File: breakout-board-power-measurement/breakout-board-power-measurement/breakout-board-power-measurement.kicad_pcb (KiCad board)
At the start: 2 copper layers, 70.6 x 40.2 mm, 83 parts, among them J1 Screw_Terminal_01x04, J2 Conn_01x09, J3 Conn_01x07, J4 Conn_01x02, U1 MCP3911A0-E-SS, U2 Si8641BA-B-IU, U3 LM317_TO-252, Y1 10M

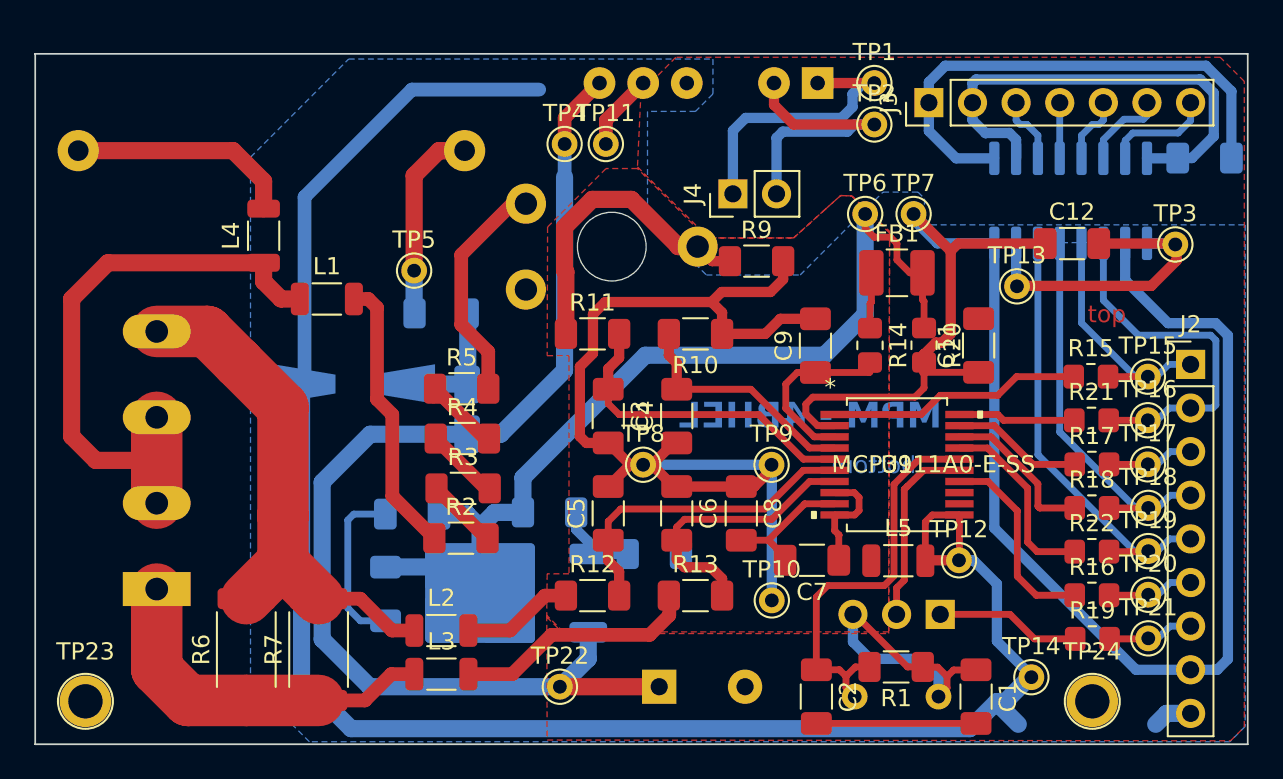
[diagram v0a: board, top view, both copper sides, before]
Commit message: Minor Fixes.
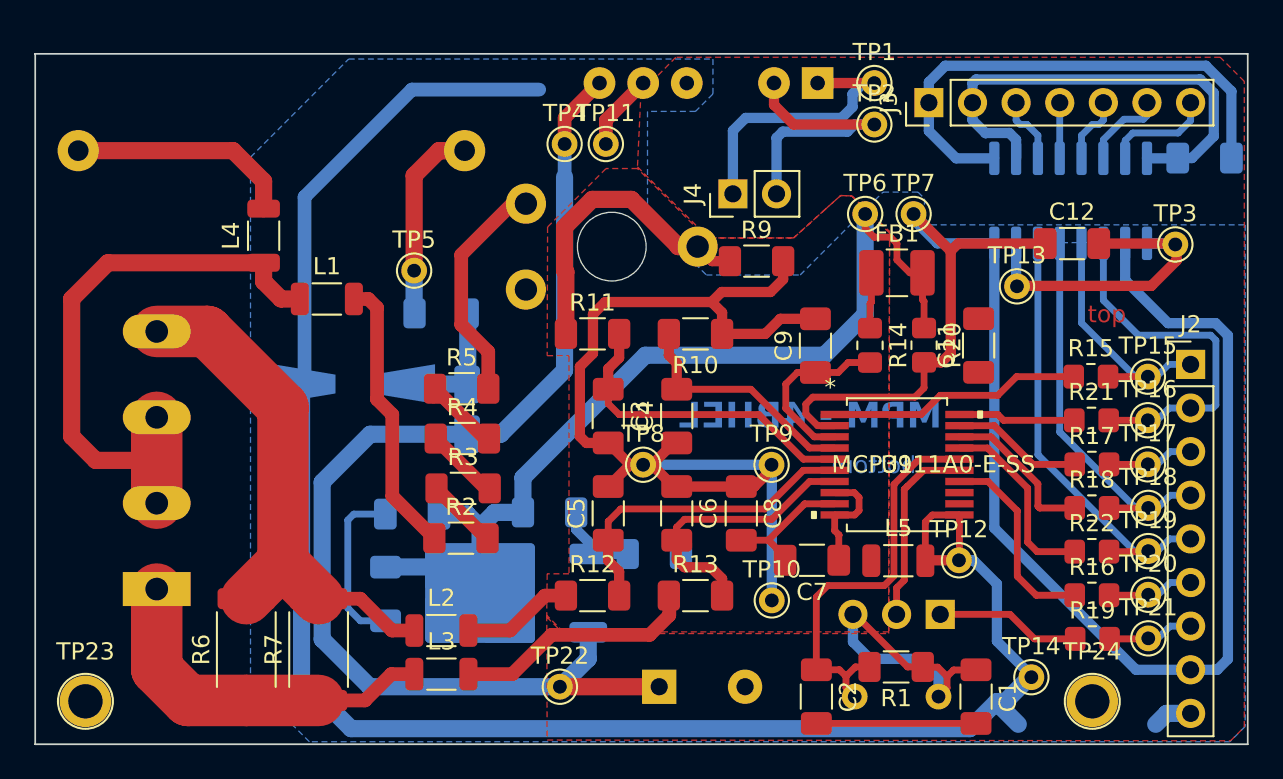
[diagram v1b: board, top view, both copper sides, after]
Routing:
- net /3V3D: track 98.8 -> 95.1 mm
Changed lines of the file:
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@@
   (segment (start 167.8432 143.5608) (end 168.402 143.002) (width 0.4) (layer "F.Cu") (net 9))
   (segment (start 162.1028 131.826) (end 162.7755 131.1533) (width 0.4) (layer "F.Cu") (net 10))
-  (segment (start 163.83 131.153298) (end 166.976701 131.153298) (width 0.4) (layer "F.Cu") (net 10))
+  (segment (start 165.736534 130.573466) (end 167.006533 130.573466) (width 0.4) (layer "F.Cu") (net 10))
+  (segment (start 165.156702 131.153298) (end 165.736534 130.573466) (width 0.4) (layer "F.Cu") (net 10))
+  (segment (start 163.83 131.153298) (end 165.156702 131.153298) (width 0.4) (layer "F.Cu") (net 10))
   (segment (start 164.9476 134.899999) (end 163.756198 134.899999) (width 0.4) (layer "F.Cu") (net 10))
   (segment (start 163.756198 134.899999) (end 162.1028 133.246601) (width 0.4) (layer "F.Cu") (net 10))
@@
   (segment (start 163.829998 131.1533) (end 163.83 131.153298) (width 0.4) (layer "F.Cu") (net 10))
   (segment (start 162.7755 131.1533) (end 163.829998 131.1533) (width 0.4) (layer "F.Cu") (net 10))
-  (segment (start 166.976701 131.153298) (end 167.006533 131.123466) (width 0.4) (layer "F.Cu") (net 10))
-  (segment (start 170.153066 130.074934) (end 170.178592 130.074934) (width 0.6) (layer "F.Cu") (net 11))
-  (segment (start 171.704 128.905) (end 171.704 124.084) (width 0.6) (layer "F.Cu") (net 11))
-  (segment (start 173.3296 131.144632) (end 170.182898 131.144632) (width 0.4) (layer "F.Cu") (net 11))
+  (segment (start 171.704 124.084) (end 171.704 130.016) (width 0.6) (layer "F.Cu") (net 11))
   (segment (start 169.6212 132.588) (end 170.153066 132.056134) (width 0.4) (layer "F.Cu") (net 11))
   (segment (start 164.9476 134.250001) (end 163.954728 134.250001) (width 0.4) (layer "F.Cu") (net 11))
+  (segment (start 170.153066 132.056134) (end 170.153066 130.5648) (width 0.4) (layer "F.Cu") (net 11))
+  (segment (start 171.704 130.016) (end 171.1552 130.5648) (width 0.6) (layer "F.Cu") (net 11))
   (segment (start 163.6776 132.588) (end 169.6212 132.588) (width 0.4) (layer "F.Cu") (net 11))
-  (segment (start 170.182898 131.144632) (end 170.153066 131.1148) (width 0.4) (layer "F.Cu") (net 11))
   (segment (start 172.1408 123.6472) (end 171.704 124.084) (width 0.6) (layer "F.Cu") (net 11))
-  (segment (start 170.840526 129.413) (end 171.196 129.413) (width 0.6) (layer "F.Cu") (net 11))
   (segment (start 163.2712 133.566473) (end 163.2712 132.9944) (width 0.4) (layer "F.Cu") (net 11))
   (segment (start 171.704 124.084) (end 169.545 121.925) (width 0.6) (layer "F.Cu") (net 11))
   (segment (start 163.954728 134.250001) (end 163.2712 133.566473) (width 0.4) (layer "F.Cu") (net 11))
   (segment (start 177.2027 123.6472) (end 172.1408 123.6472) (width 0.6) (layer "F.Cu") (net 11))
-  (segment (start 170.153066 131.1148) (end 170.153066 130.074934) (width 0.6) (layer "F.Cu") (net 11))
-  (segment (start 171.196 129.413) (end 171.704 128.905) (width 0.6) (layer "F.Cu") (net 11))
-  (segment (start 170.178592 130.074934) (end 170.840526 129.413) (width 0.6) (layer "F.Cu") (net 11))
   (segment (start 163.2712 132.9944) (end 163.6776 132.588) (width 0.4) (layer "F.Cu") (net 11))
-  (segment (start 170.153066 132.056134) (end 170.153066 131.1148) (width 0.4) (layer "F.Cu") (net 11))
+  (segment (start 171.1552 130.5648) (end 170.153066 130.5648) (width 0.6) (layer "F.Cu") (net 11))
   (segment (start 170.9278 123.633) (end 174.244 123.633) (width 0.6) (layer "B.Cu") (net 11))
   (segment (start 182.499 148.463) (end 174.244 140.208) (width 0.6) (layer "B.Cu") (net 11))
   (segment (start 187.8472 147.8392) (end 187.2234 148.463) (width 0.6) (layer "B.Cu") (net 11))
-  (segment (start 169.5704 121.4628) (end 169.5704 122.2756) (width 0.6) (layer "B.Cu") (net 11))
   (segment (start 181.864 125.7808) (end 184.3644 128.2812) (width 0.6) (layer "B.Cu") (net 11))
   (segment (start 169.5704 122.2756) (end 170.9278 123.633) (width 0.6) (layer "B.Cu") (net 11))
@@
   (segment (start 134.9 144.325) (end 137.325 144.325) (width 0.8) (layer "F.Cu") (net 36))
   (segment (start 132.825 142.05) (end 132.825 142.19) (width 3) (layer "F.Cu") (net 36))
-  (segment (start 130.225 130.575) (end 132.825 133.175) (width 3) (layer "F.Cu") (net 36))
+  (segment (start 128.414 128.764) (end 132.825 133.175) (width 3) (layer "F.Cu") (net 36))
   (segment (start 132.825 142.25) (end 134.9 144.325) (width 3) (layer "F.Cu") (net 36))
   (segment (start 139.177 146.177) (end 140.475 146.177) (width 0.8) (layer "F.Cu") (net 36))
-  (segment (start 132.825 133.175) (end 132.825 139.5) (width 3) (layer "F.Cu") (net 36))
-  (segment (start 132.825 139.5) (end 132.825 142.05) (width 3) (layer "F.Cu") (net 36))
+  (segment (start 132.825 133.175) (end 132.825 142.05) (width 3) (layer "F.Cu") (net 36))
   (segment (start 132.825 142.19) (end 130.69 144.325) (width 3) (layer "F.Cu") (net 36))
   (segment (start 132.825 142.05) (end 132.825 142.25) (width 3) (layer "F.Cu") (net 36))
   (segment (start 137.325 144.325) (end 139.177 146.177) (width 0.8) (layer "F.Cu") (net 36))
-  (segment (start 128.414 128.764) (end 130.225 130.575) (width 3) (layer "F.Cu") (net 36))
   (segment (start 141.638 140.8) (end 139.192 138.354) (width 0.8) (layer "F.Cu") (net 37))
   (segment (start 137.795 126.873) (end 136.957 126.873) (width 0.8) (layer "F.Cu") (net 37))
@@
   (segment (start 152.9 141.725) (end 150.605 141.725) (width 0.6) (layer "B.Cu") (net 50))
   (segment (start 150.605 141.725) (end 150.6 141.72) (width 0.6) (layer "B.Cu") (net 50))
-  (segment (start 152.895 141.72) (end 152.9 141.725) (width 0.4) (layer "B.Cu") (net 50))
   (segment (start 167.259 116.713) (end 162.56 116.713) (width 0.6) (layer "F.Cu") (net 53))
   (segment (start 162.56 116.713) (end 161.417 115.57) (width 0.6) (layer "F.Cu") (net 53))
